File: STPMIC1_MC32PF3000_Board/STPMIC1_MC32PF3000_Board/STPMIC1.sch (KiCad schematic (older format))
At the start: 48 parts, among them U3 STPMIC1

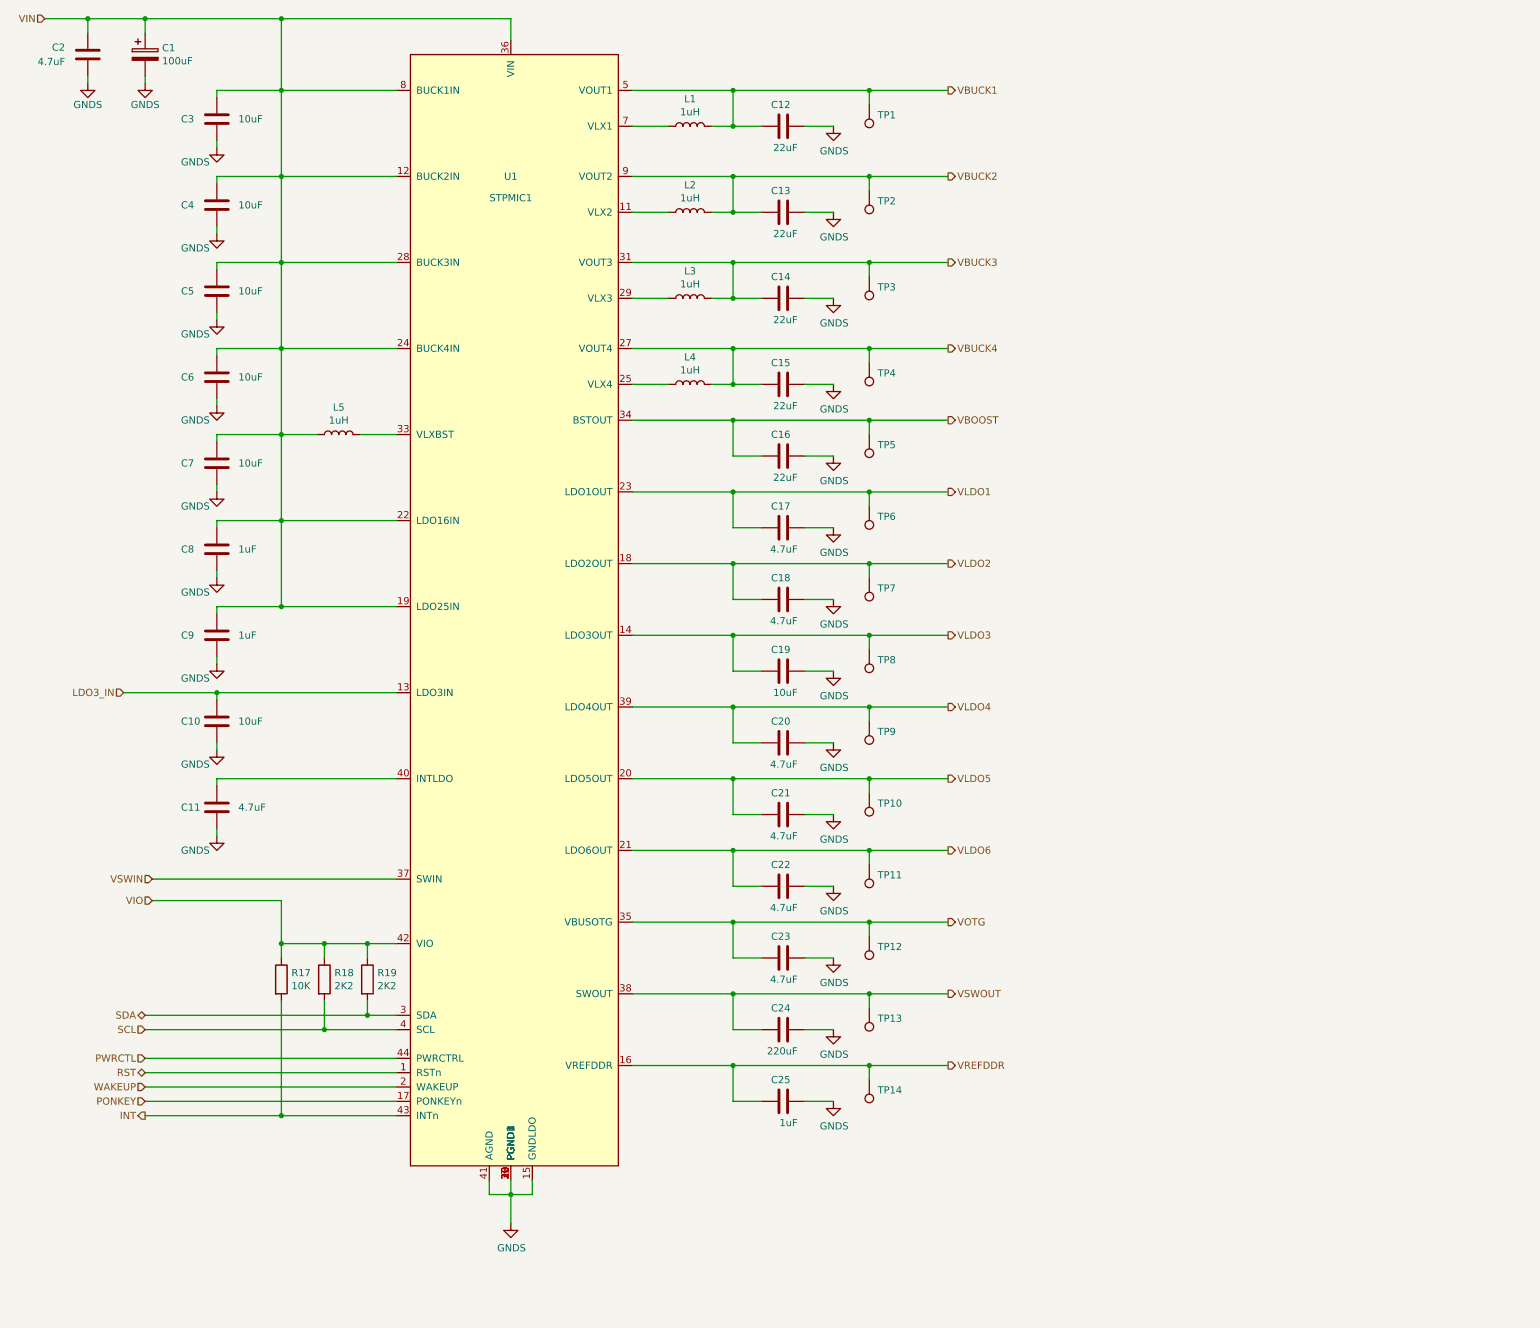
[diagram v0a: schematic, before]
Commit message: updated schema document
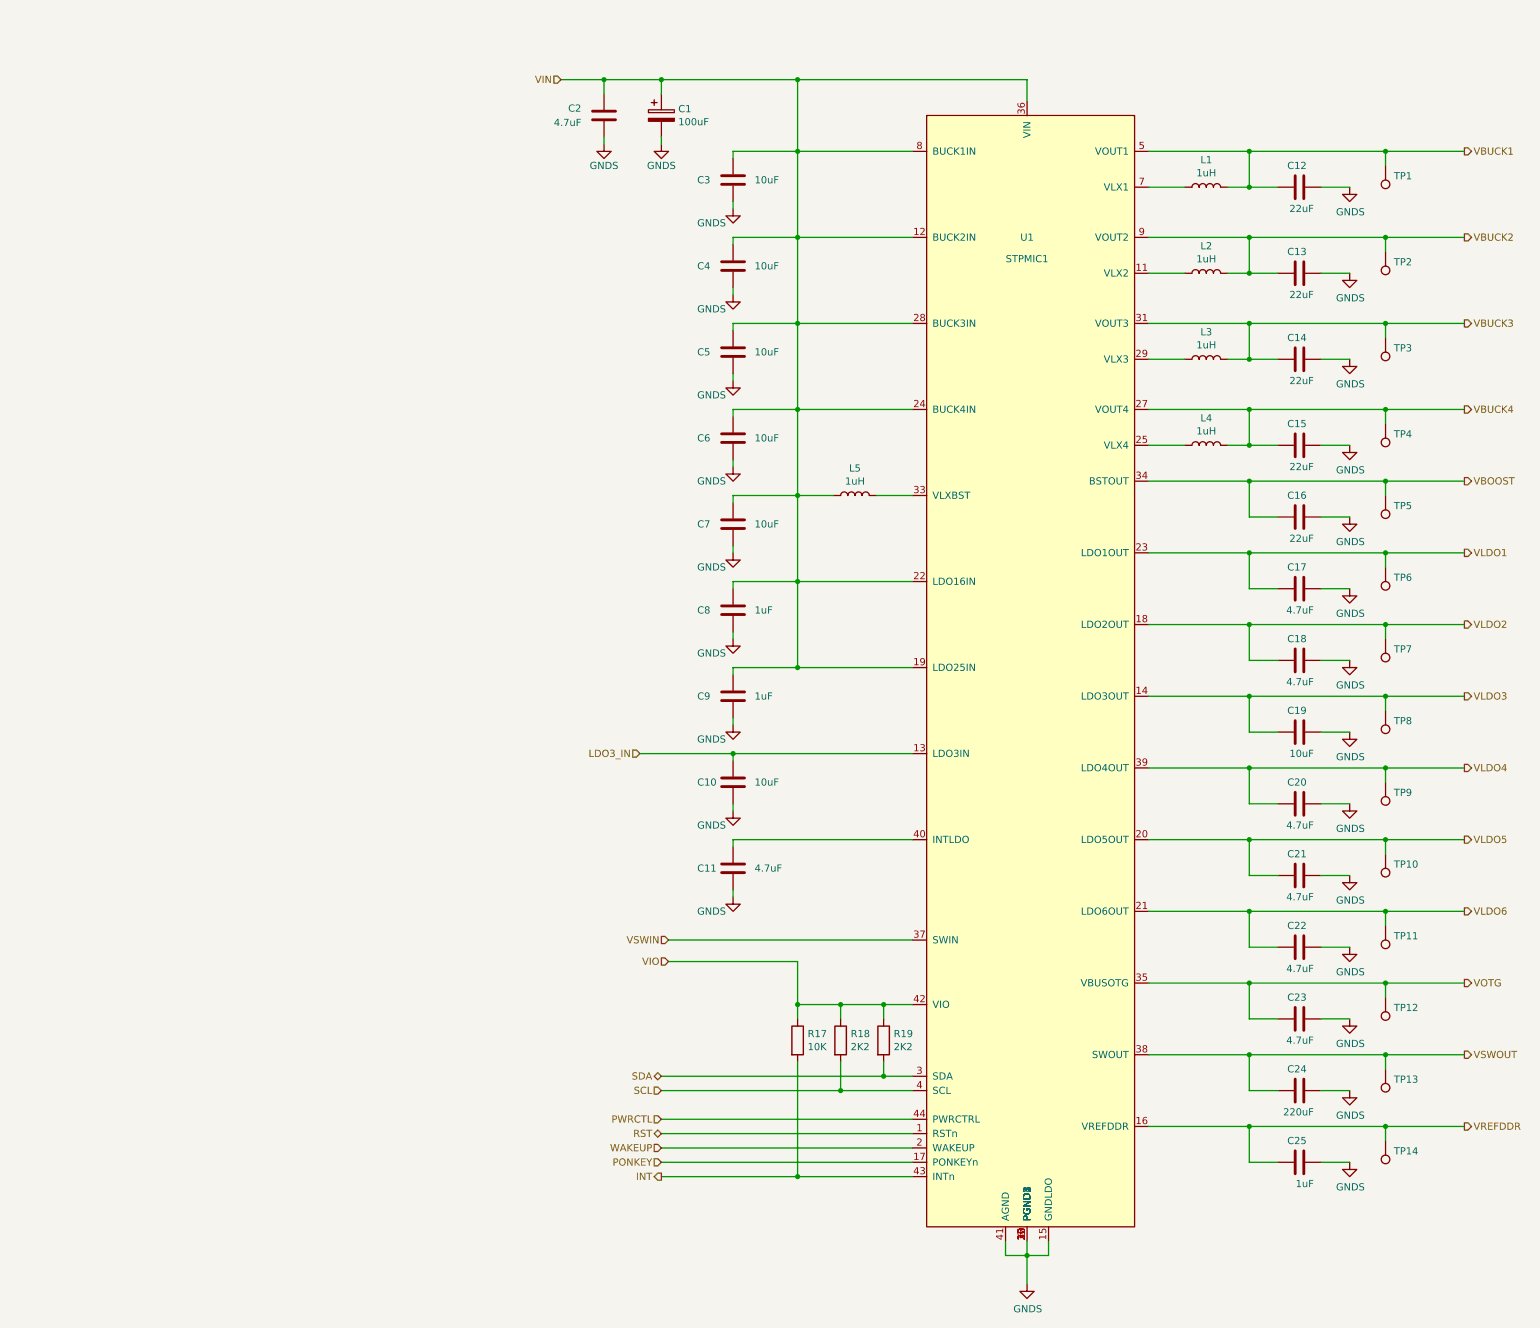
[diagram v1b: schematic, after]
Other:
- moved on the sheet: C1, C10, C11, C12, C13, C14, C15, C16, C17, C18, C19, C2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

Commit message: Completed RevA layout
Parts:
- C11, C12, C13, C14, C15: footprint Capacitor_SMD:C_0603_1608Metric_Pad1.08x0.95mm_HandSolder -> Capacitor_SMD:C_0805_2012Metric_Pad1.18x1.45mm_HandSolder; MfrNum (none) -> CL21A226MPQNNNE; Type (none) -> CAP CER 22uF 25V 20% X5R 0805
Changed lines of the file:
@@
 F 0 "C12" V 9750 2175 50  0000 L CNN
 F 1 "22uF" V 9450 2125 50  0000 L CNN
-F 2 "Capacitor_SMD:C_0603_1608Metric_Pad1.08x0.95mm_HandSolder" H 9638 2075 50  0001 C CNN
+F 2 "Capacitor_SMD:C_0805_2012Metric_Pad1.18x1.45mm_HandSolder" H 9638 2075 50  0001 C CNN
 F 3 "~" H 9600 2225 50  0001 C CNN
+F 4 "CL21A226MPQNNNE" H 9600 2225 50  0001 C CNN "MfrNum"
+F 5 "CAP CER 22uF 25V 20% X5R 0805" H 9600 2225 50  0001 C CNN "Type"
 	1    9600 2225
 	0    -1   -1   0
@@
 F 0 "C13" V 9750 2775 50  0000 L CNN
 F 1 "22uF" V 9450 2725 50  0000 L CNN
-F 2 "Capacitor_SMD:C_0603_1608Metric_Pad1.08x0.95mm_HandSolder" H 9638 2675 50  0001 C CNN
+F 2 "Capacitor_SMD:C_0805_2012Metric_Pad1.18x1.45mm_HandSolder" H 9638 2675 50  0001 C CNN
 F 3 "~" H 9600 2825 50  0001 C CNN
+F 4 "CL21A226MPQNNNE" H 9600 2825 50  0001 C CNN "MfrNum"
+F 5 "CAP CER 22uF 25V 20% X5R 0805" H 9600 2825 50  0001 C CNN "Type"
 	1    9600 2825
 	0    -1   -1   0
@@
 F 0 "C14" V 9750 3375 50  0000 L CNN
 F 1 "22uF" V 9450 3325 50  0000 L CNN
-F 2 "Capacitor_SMD:C_0603_1608Metric_Pad1.08x0.95mm_HandSolder" H 9638 3275 50  0001 C CNN
+F 2 "Capacitor_SMD:C_0805_2012Metric_Pad1.18x1.45mm_HandSolder" H 9638 3275 50  0001 C CNN
 F 3 "~" H 9600 3425 50  0001 C CNN
+F 4 "CL21A226MPQNNNE" H 9600 3425 50  0001 C CNN "MfrNum"
+F 5 "CAP CER 22uF 25V 20% X5R 0805" H 9600 3425 50  0001 C CNN "Type"
 	1    9600 3425
 	0    -1   -1   0
@@
 F 0 "C15" V 9750 3975 50  0000 L CNN
 F 1 "22uF" V 9450 3925 50  0000 L CNN
-F 2 "Capacitor_SMD:C_0603_1608Metric_Pad1.08x0.95mm_HandSolder" H 9638 3875 50  0001 C CNN
+F 2 "Capacitor_SMD:C_0805_2012Metric_Pad1.18x1.45mm_HandSolder" H 9638 3875 50  0001 C CNN
 F 3 "~" H 9600 4025 50  0001 C CNN
+F 4 "CL21A226MPQNNNE" H 9600 4025 50  0001 C CNN "MfrNum"
+F 5 "CAP CER 22uF 25V 20% X5R 0805" H 9600 4025 50  0001 C CNN "Type"
 	1    9600 4025
 	0    -1   -1   0
@@
 F 0 "C16" V 9750 4475 50  0000 L CNN
 F 1 "22uF" V 9450 4425 50  0000 L CNN
-F 2 "Capacitor_SMD:C_0603_1608Metric_Pad1.08x0.95mm_HandSolder" H 9638 4375 50  0001 C CNN
+F 2 "Capacitor_SMD:C_0805_2012Metric_Pad1.18x1.45mm_HandSolder" H 9638 4375 50  0001 C CNN
 F 3 "~" H 9600 4525 50  0001 C CNN
+F 4 "CL21A226MPQNNNE" H 9600 4525 50  0001 C CNN "MfrNum"
+F 5 "CAP CER 22uF 25V 20% X5R 0805" H 9600 4525 50  0001 C CNN "Type"
 	1    9600 4525
 	0    -1   -1   0

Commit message: updated RevA Layout
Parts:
- C10, C16, C17, C18, C20, C21, C24, C7, C8, C9: footprint Capacitor_SMD:C_0603_1608Metric_Pad1.08x0.95mm_HandSolder -> Capacitor_SMD:C_0805_2012Metric_Pad1.18x1.45mm_HandSolder
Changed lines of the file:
@@
 F 0 "C17" V 9750 4975 50  0000 L CNN
 F 1 "4.7uF" V 9450 4925 50  0000 L CNN
-F 2 "Capacitor_SMD:C_0603_1608Metric_Pad1.08x0.95mm_HandSolder" H 9638 4875 50  0001 C CNN
+F 2 "Capacitor_SMD:C_0805_2012Metric_Pad1.18x1.45mm_HandSolder" H 9638 4875 50  0001 C CNN
 F 3 "~" H 9600 5025 50  0001 C CNN
 	1    9600 5025
@@
 F 0 "C18" V 9750 5475 50  0000 L CNN
 F 1 "4.7uF" V 9450 5425 50  0000 L CNN
-F 2 "Capacitor_SMD:C_0603_1608Metric_Pad1.08x0.95mm_HandSolder" H 9638 5375 50  0001 C CNN
+F 2 "Capacitor_SMD:C_0805_2012Metric_Pad1.18x1.45mm_HandSolder" H 9638 5375 50  0001 C CNN
 F 3 "~" H 9600 5525 50  0001 C CNN
 	1    9600 5525
@@
 F 0 "C21" V 9750 6975 50  0000 L CNN
 F 1 "4.7uF" V 9450 6925 50  0000 L CNN
-F 2 "Capacitor_SMD:C_0603_1608Metric_Pad1.08x0.95mm_HandSolder" H 9638 6875 50  0001 C CNN
+F 2 "Capacitor_SMD:C_0805_2012Metric_Pad1.18x1.45mm_HandSolder" H 9638 6875 50  0001 C CNN
 F 3 "~" H 9600 7025 50  0001 C CNN
 	1    9600 7025
@@
 F 0 "C22" V 9750 7475 50  0000 L CNN
 F 1 "4.7uF" V 9450 7425 50  0000 L CNN
-F 2 "Capacitor_SMD:C_0603_1608Metric_Pad1.08x0.95mm_HandSolder" H 9638 7375 50  0001 C CNN
+F 2 "Capacitor_SMD:C_0805_2012Metric_Pad1.18x1.45mm_HandSolder" H 9638 7375 50  0001 C CNN
 F 3 "~" H 9600 7525 50  0001 C CNN
 	1    9600 7525
@@
 F 0 "C19" V 9750 5975 50  0000 L CNN
 F 1 "10uF" V 9450 5925 50  0000 L CNN
-F 2 "Capacitor_SMD:C_0603_1608Metric_Pad1.08x0.95mm_HandSolder" H 9638 5875 50  0001 C CNN
+F 2 "Capacitor_SMD:C_0805_2012Metric_Pad1.18x1.45mm_HandSolder" H 9638 5875 50  0001 C CNN
 F 3 "~" H 9600 6025 50  0001 C CNN
 	1    9600 6025
@@
 F 0 "C25" V 9750 8975 50  0000 L CNN
 F 1 "1uF" V 9450 8925 50  0000 L CNN
-F 2 "Capacitor_SMD:C_0603_1608Metric_Pad1.08x0.95mm_HandSolder" H 9638 8875 50  0001 C CNN
+F 2 "Capacitor_SMD:C_0805_2012Metric_Pad1.18x1.45mm_HandSolder" H 9638 8875 50  0001 C CNN
 F 3 "~" H 9600 9025 50  0001 C CNN
 	1    9600 9025
@@
 F 0 "C8" H 5400 5175 50  0000 L CNN
 F 1 "1uF" H 5800 5175 50  0000 L CNN
-F 2 "Capacitor_SMD:C_0603_1608Metric_Pad1.08x0.95mm_HandSolder" H 5688 5025 50  0001 C CNN
+F 2 "Capacitor_SMD:C_0805_2012Metric_Pad1.18x1.45mm_HandSolder" H 5688 5025 50  0001 C CNN
 F 3 "~" H 5650 5175 50  0001 C CNN
 	1    5650 5175
@@
 F 0 "C9" H 5400 5775 50  0000 L CNN
 F 1 "1uF" H 5800 5775 50  0000 L CNN
-F 2 "Capacitor_SMD:C_0603_1608Metric_Pad1.08x0.95mm_HandSolder" H 5688 5625 50  0001 C CNN
+F 2 "Capacitor_SMD:C_0805_2012Metric_Pad1.18x1.45mm_HandSolder" H 5688 5625 50  0001 C CNN
 F 3 "~" H 5650 5775 50  0001 C CNN
 	1    5650 5775
@@
 F 0 "C10" H 5400 6375 50  0000 L CNN
 F 1 "10uF" H 5800 6375 50  0000 L CNN
-F 2 "Capacitor_SMD:C_0603_1608Metric_Pad1.08x0.95mm_HandSolder" H 5688 6225 50  0001 C CNN
+F 2 "Capacitor_SMD:C_0805_2012Metric_Pad1.18x1.45mm_HandSolder" H 5688 6225 50  0001 C CNN
 F 3 "~" H 5650 6375 50  0001 C CNN
 	1    5650 6375
@@
 F 0 "C11" H 5400 6975 50  0000 L CNN
 F 1 "4.7uF" H 5800 6975 50  0000 L CNN
-F 2 "Capacitor_SMD:C_0603_1608Metric_Pad1.08x0.95mm_HandSolder" H 5688 6825 50  0001 C CNN
+F 2 "Capacitor_SMD:C_0805_2012Metric_Pad1.18x1.45mm_HandSolder" H 5688 6825 50  0001 C CNN
 F 3 "~" H 5650 6975 50  0001 C CNN
 	1    5650 6975

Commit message: Completed RevA
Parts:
- C1, C19, C22: footprint Capacitor_SMD:C_0603_1608Metric_Pad1.08x0.95mm_HandSolder -> Capacitor_SMD:C_0805_2012Metric_Pad1.18x1.45mm_HandSolder; LCSC (none) -> C1779
- C10, C16, C17, C20, C21: LCSC (none) -> C1779
- C11, C12, C13, C14, C15: LCSC (none) -> C45783
- C18, C9: LCSC (none) -> C15850
- C2, C3, C4, C5, C6: footprint Capacitor_SMD:C_0603_1608Metric_Pad1.08x0.95mm_HandSolder -> Capacitor_SMD:C_0805_2012Metric_Pad1.18x1.45mm_HandSolder; LCSC (none) -> C15850
- C24, C7, C8: LCSC (none) -> C28323
- C25: footprint Capacitor_SMD:C_Elec_4x5.4 -> Capacitor_SMD:C_Elec_6.3x7.7; LCSC (none) -> C127971
- L1, L2, L3, L4, L5: Mouser (none) -> 81-DFE252012P-1R0MP2; Type (none) -> IND PWR 1.0μH, 3.5A, 42mΩ 1008
- R1, R2: LCSC (none) -> C17520
- R3: LCSC (none) -> C17414
- U3: MfrNum (none) -> STPMIC1APQR; Mouser (none) -> 511-STPMIC1APQR
